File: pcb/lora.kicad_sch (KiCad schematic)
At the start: 57 parts, among them J1 Conn_01x04, J11 Conn_Coaxial, J2 5V, J3 Temp, J5 Temp, J6 VDD, J7 UART, J9 I2C, Q2 AO3401A, Q3 AO3401A, Q5 AO3401A, SW1 RESET, SW2 PJ, U1 ME2108C50M5G, U2 ESP32-WROOM-32D, U3 2460, U4 RFM95W-868S2

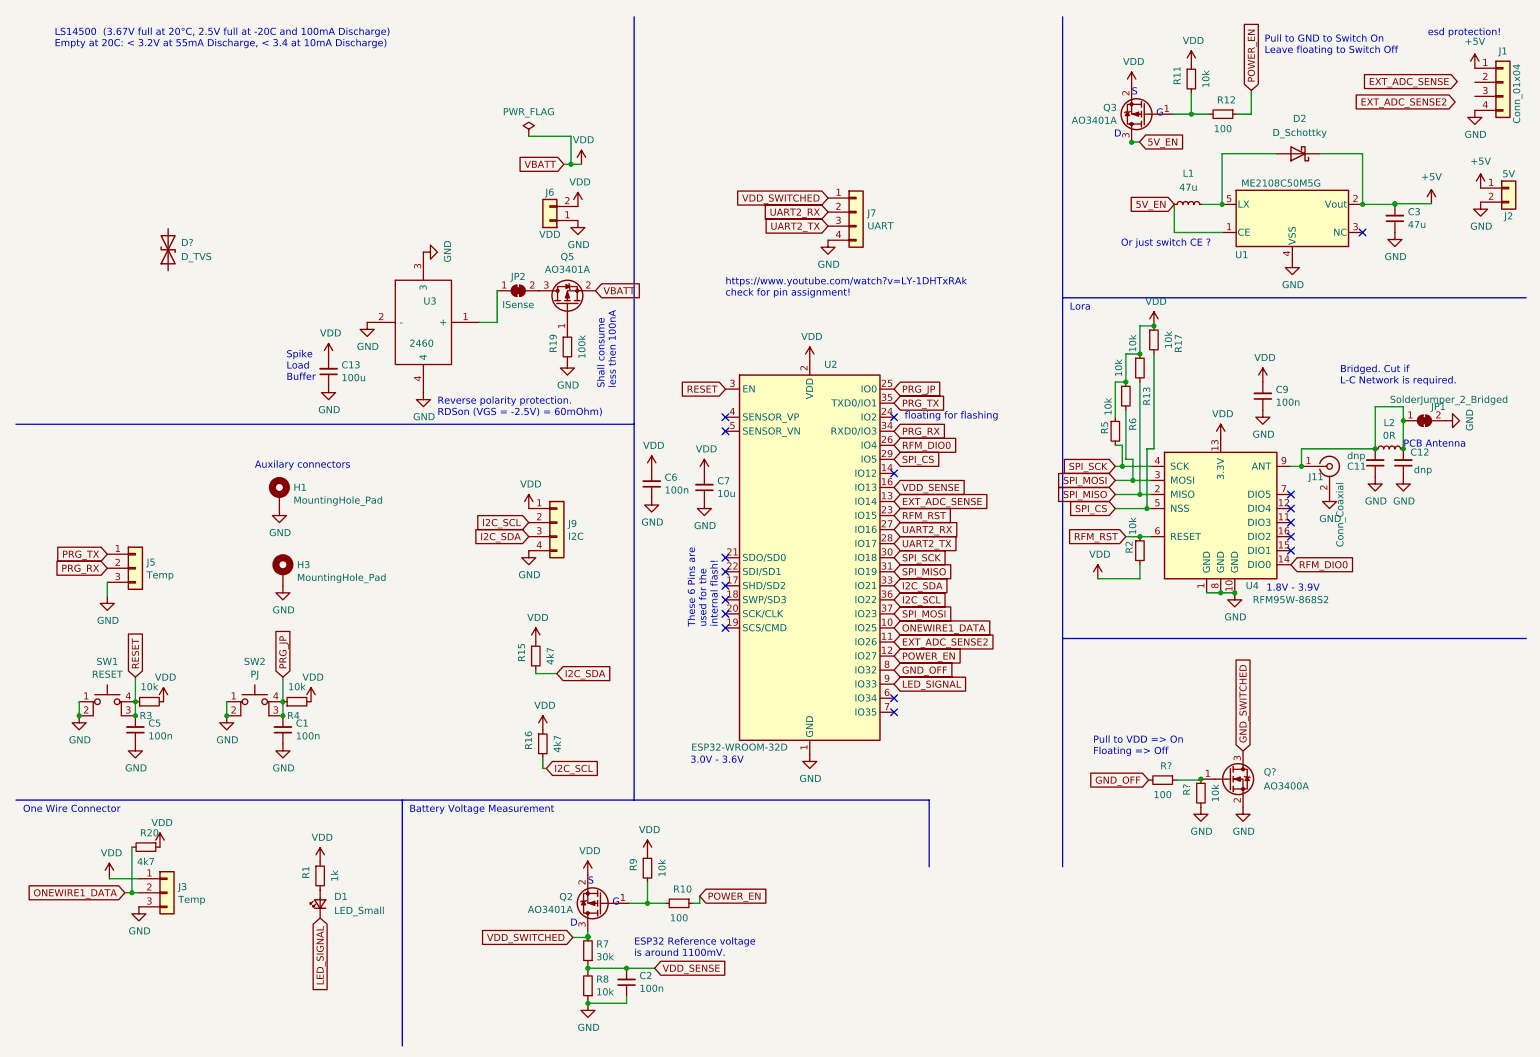
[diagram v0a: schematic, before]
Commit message: schematic finalized
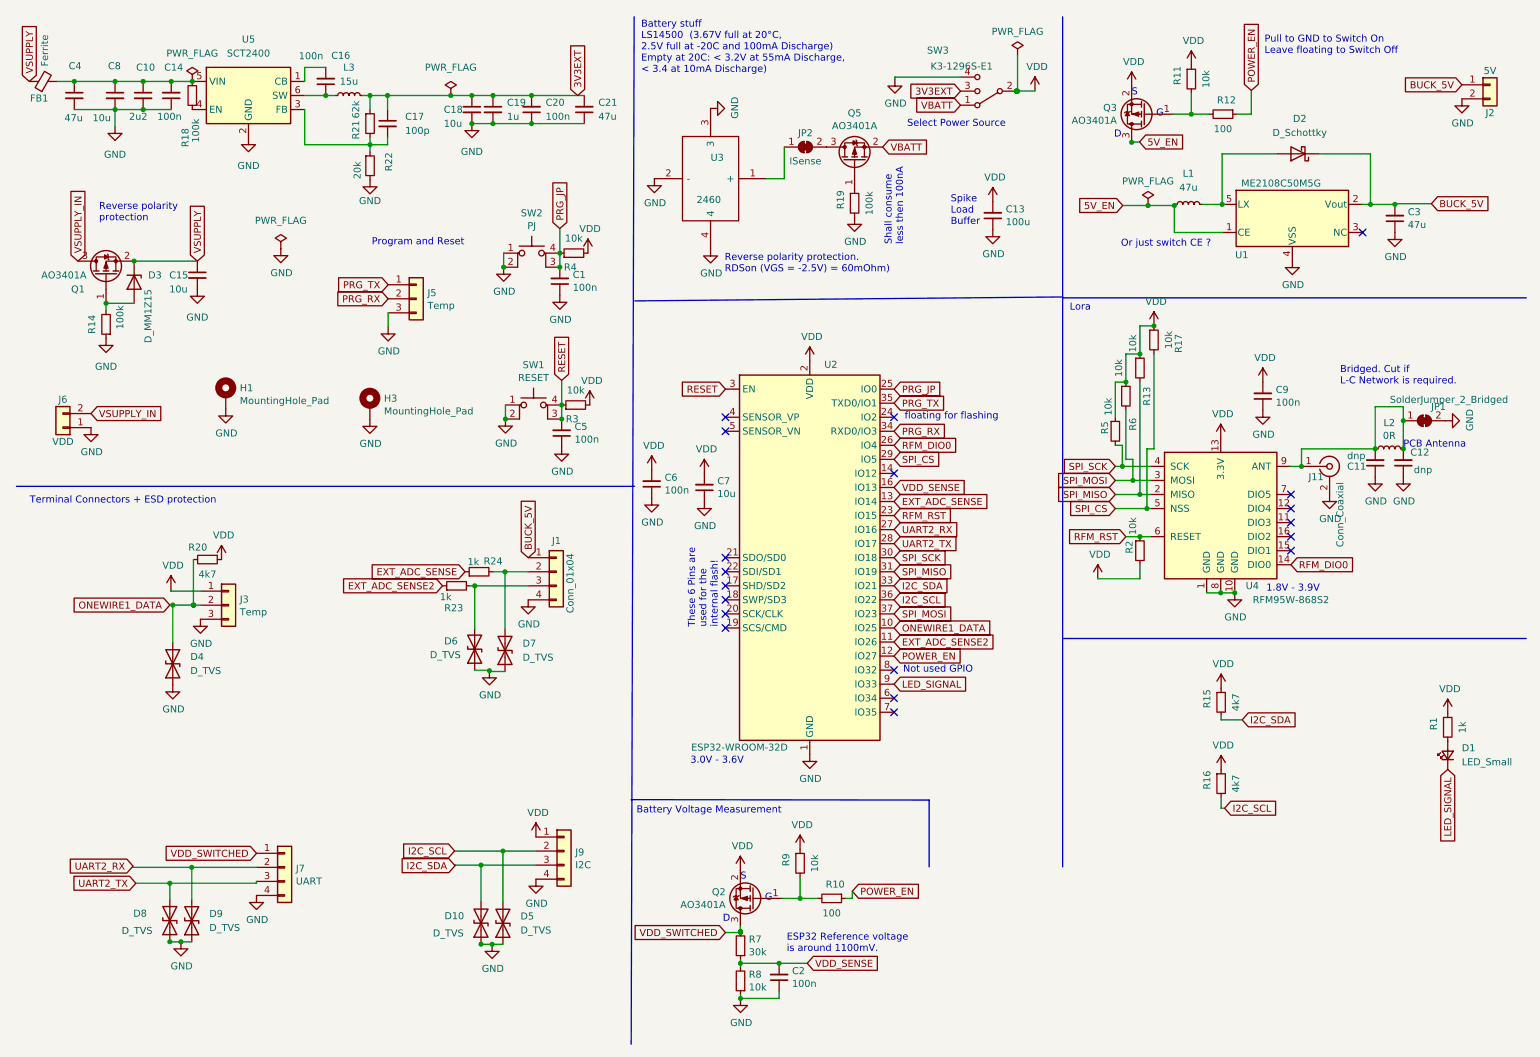
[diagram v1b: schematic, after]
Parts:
- removed Q?: AO3400A, Package_TO_SOT_SMD:SOT-23, symbol Transistor_FET:AO3400A
- removed R?: 100, Resistor_SMD:R_0603_1608Metric, symbol Device:R_Small
- removed R?: 10k, Capacitor_SMD:C_0603_1608Metric, symbol Device:R_Small
- added C10: 2u2, Capacitor_SMD:C_0805_2012Metric, symbol Device:C_Small
- added C14, C16, C20: 100n, Capacitor_SMD:C_0603_1608Metric, symbol Device:C_Small
- added C15, C18, C8: 10u, Capacitor_SMD:C_0805_2012Metric, symbol Device:C_Small
- added C17: 100p, Capacitor_SMD:C_0603_1608Metric, symbol Device:C_Small
- added C19: 1u, Capacitor_SMD:C_0603_1608Metric, symbol Device:C_Small
- added C21, C4: 47u, Capacitor_SMD:C_1206_3216Metric, symbol Device:C_Small
- added D10, D4, D6, D7, D8, D9: D_TVS, Diode_SMD:D_0402_1005Metric, symbol Device:D_TVS
- added D3: D_MM1Z15, Diode_SMD:D_SOD-123, symbol Device:D_Zener
- added FB1: Ferrite, Inductor_SMD:L_0805_2012Metric, symbol Device:FerriteBead_Small
- added L3: 15u, OWN_PARTS:SLO0630H, symbol Device:L_Small
- added Q1: AO3401A, Package_TO_SOT_SMD:SOT-23, symbol Transistor_FET:AO3401A
- added R14, R18: 100k, Resistor_SMD:R_0603_1608Metric, symbol Device:R_Small
- added R21: 62k, Resistor_SMD:R_0603_1608Metric, symbol Device:R_Small
- added R22: 20k, Resistor_SMD:R_0603_1608Metric, symbol Device:R_Small
- added R23, R24: 1k, Capacitor_SMD:C_0603_1608Metric, symbol Device:R_Small
- added SW3: K3-1296S-E1, OWN_Parts_:K3-1296S-E1, symbol OWN_Parts_:K3-1296S-E1
- added U5: SCT2400, Package_TO_SOT_SMD:TSOT-23-6, symbol lv2842x:LV2842X
- J1: footprint (none) -> TerminalBlock_TE-Connectivity:TerminalBlock_TE_282834-4_1x04_P2.54mm_Horizontal
- J3: footprint Connector_PinHeader_2.54mm:PinHeader_1x03_P2.54mm_Horizontal -> TerminalBlock_TE-Connectivity:TerminalBlock_TE_282834-3_1x03_P2.54mm_Horizontal
- J6: footprint Connector_PinHeader_2.54mm:PinHeader_1x02_P2.54mm_Vertical -> TerminalBlock_TE-Connectivity:TerminalBlock_TE_282834-2_1x02_P2.54mm_Horizontal
- J7, J9: footprint Connector_PinHeader_2.54mm:PinHeader_1x04_P2.54mm_Vertical -> TerminalBlock_TE-Connectivity:TerminalBlock_TE_282834-4_1x04_P2.54mm_Horizontal
- U3: footprint SamacSys_Parts:2460 -> 2460
- gave numbers to parts that had none: 1
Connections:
- net EXT_ADC_SENSE: now also R24.1
- net EXT_ADC_SENSE2: now also R23.1
- net GND: now also D5.1 (A1), C10.2, C14.1, C15.2, C18.2, C19.2, C20.1, C21.1, C4.2, C8.2, D10.1 (A1), D4.1 (A1), D6.1 (A1), D7.1 (A1), D8.1 (A1), D9.1 (A1), R14.1, R22.2, SW3.4, U5.2 (GND)
- net I2C_SCL: now also D5.2 (A2)
- net I2C_SDA: now also D10.2 (A2)
- net ONEWIRE1_DATA: now also D4.2 (A2)
- net UART2_RX: now also D9.2 (A2)
- net UART2_TX: now also D8.2 (A2)
- net VDD: now also SW3.2; no longer J6.2 (Pin_2), Q5.2 (S)
- net at J1.2 (Pin_2): now also D7.2 (A2), R24.2
- net at J1.3 (Pin_3): now also D6.2 (A2), R23.2
- net +5V renamed BUCK_5V
- net GND_OFF: no longer names the net of U2.8 (IO32)
- new net: C10.1, C14.2, C4.1, C8.1, FB1.2, R18.2, U5.5 (VIN)
- new net: C17.2, R21.2, R22.1, U5.3 (FB)
- new net: D3.2 (A), Q1.1 (G), R14.2
- new net: R18.1, U5.4 (EN)
- new net: C16.1, L3.1, U5.6 (SW)
- new net: C16.2, U5.1 (CB)
- new net 3V3EXT: C17.1, C18.1, C19.1, C20.2, C21.2, L3.2, R21.1, SW3.3
- new net VBATT: Q5.2 (S), SW3.1
- new net VSUPPLY: C15.1, D3.1 (K), FB1.1, Q1.2 (S)
- new net VSUPPLY_IN: J6.2 (Pin_2), Q1.3 (D)
- no-connect marks 18 -> 19
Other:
- note added: "Battery stuff LS14500 (3.67V full at 20°C, 2.5V full at -20C and 100mA Discharge) Empty at 20C: < 3.2V at 55mA Discharge, < 3.4 at 10mA Discharge)"
- note added: "Not used GPIO"
- note added: "Program and Reset"
- note added: "Reverse polarity protection"
- note added: "Select Power Source"
- note added: "Terminal Connectors + ESD protection"
- note removed: "Auxilary connectors"
- note removed: "LS14500 (3.67V full at 20°C, 2.5V full at -20C and 100mA Discharge) Empty at 20C: < 3.2V at 55mA Discharge, < 3.4 at 10mA Discharge)"
- note removed: "One Wire Connector"
- note removed: "Pull to VDD => On Floating => Off"
- note removed: "esd protection!"
- note removed: "https://www.youtube.com/watch?v=LY-1DHTxRAk check for pin assignment!"
- moved on the sheet: C1, C13, C2, C5, D1, D5, H1, H3, J1, J2, J3, J5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
